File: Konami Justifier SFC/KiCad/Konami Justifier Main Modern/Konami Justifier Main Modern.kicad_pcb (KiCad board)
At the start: 4 copper layers, 25.2 x 50 mm, 20 parts, among them J1 RJ12, U1 74VHC9164FT

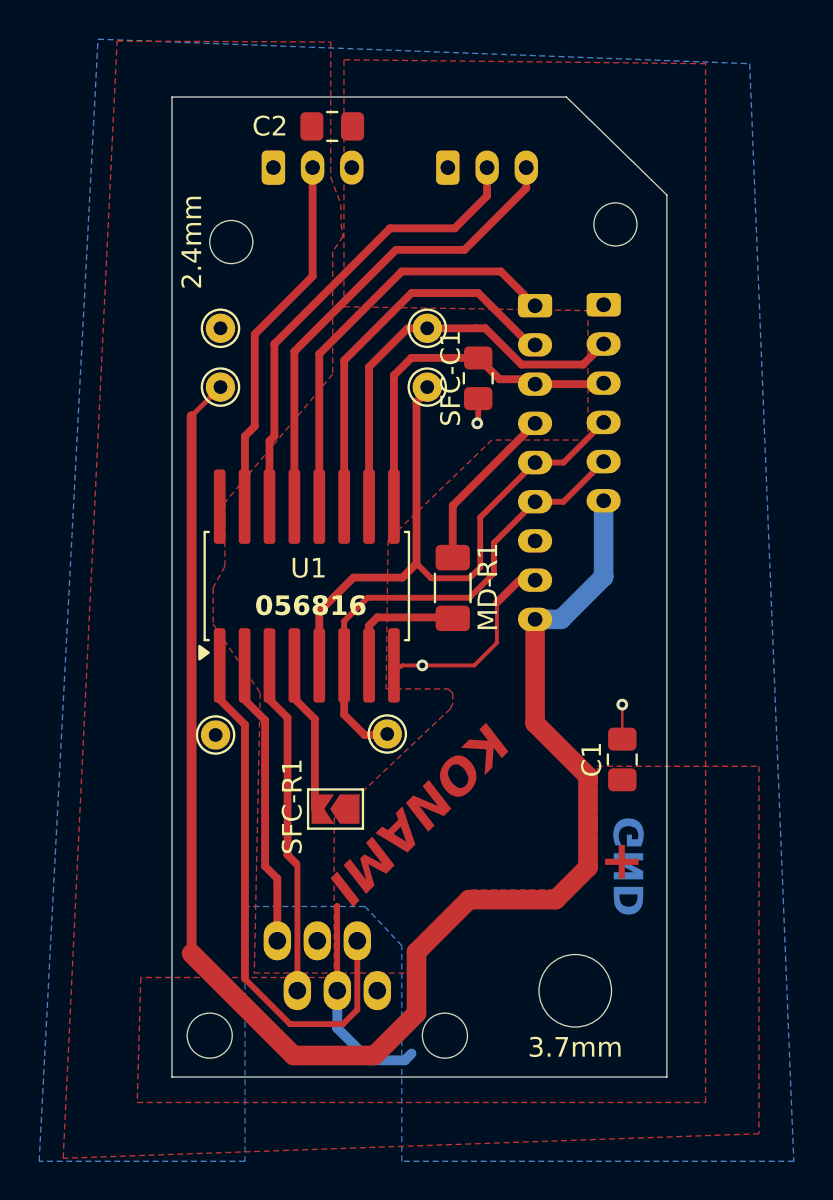
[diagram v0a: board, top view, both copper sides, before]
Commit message: Add files via upload
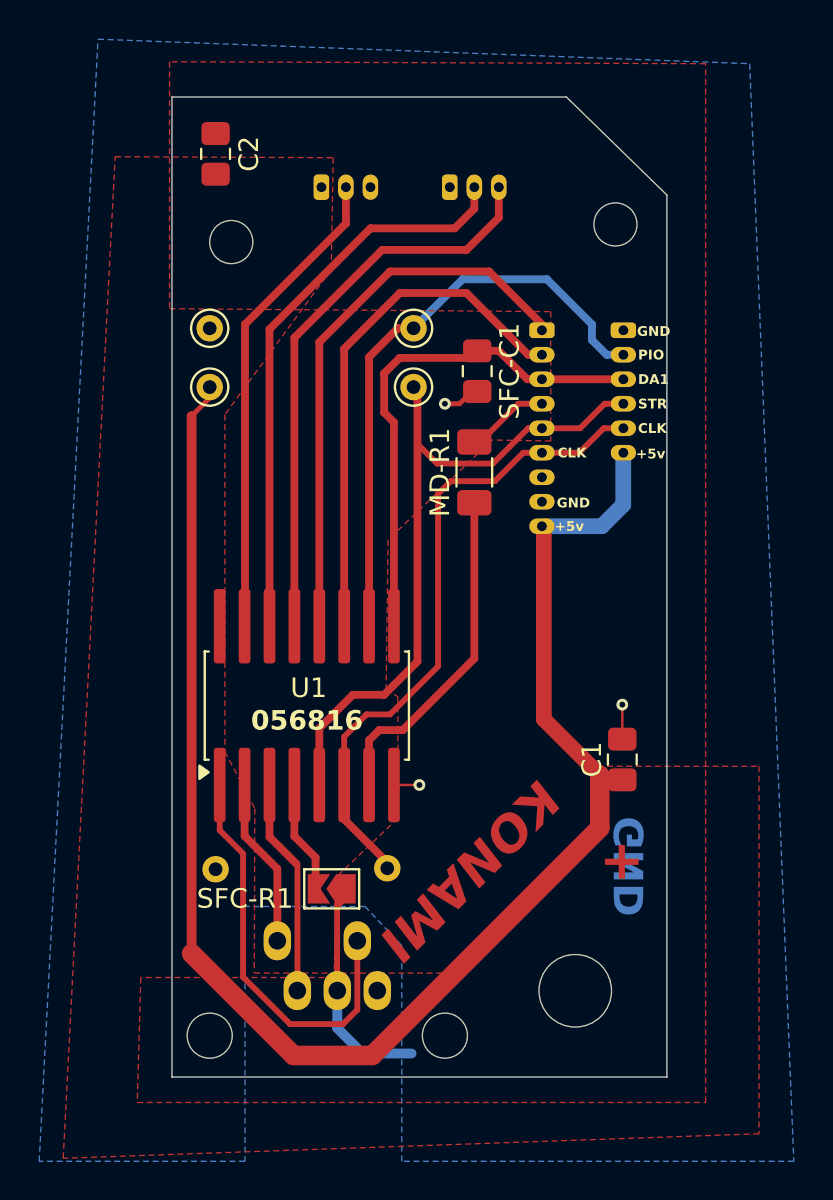
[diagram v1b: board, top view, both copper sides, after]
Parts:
- J_BTN1, J_IR1: footprint Connector_JST:JST_PH_B3B-PH-K_1x03_P2.00mm_Vertical -> Connector_Molex:Molex_PicoBlade_53048-0310_1x03_P1.25mm_Horizontal
- MD1: footprint Connector_JST:JST_PH_B9B-PH-K_1x09_P2.00mm_Vertical -> Connector_Molex:Molex_PicoBlade_53047-0910_1x09_P1.25mm_Vertical
- SFC-TP5, SFC-TP6: moved to B.Cu
- SFC1: footprint Connector_JST:JST_PH_B6B-PH-K_1x06_P2.00mm_Vertical -> Connector_Molex:Molex_PicoBlade_53047-0610_1x06_P1.25mm_Vertical
- moved SFC-TP5 6.85 mm to (142.0, 116.1), turned to 180 degrees
- moved SFC-TP6 6.85 mm to (150.8, 116.0), turned to 180 degrees
- moved C2 6.11 mm to (142.0, 79.6), turned to 90 degrees
- moved U1 6.10 mm to (146.7, 107.8)
- moved MD-R1 6.00 mm to (155.2, 95.8)
- moved SFC-R1 4.07 mm to (147.9, 117.1)
- moved J_IR1 2.65 mm to (147.4, 81.3)
- moved SFC1 1.64 mm to (162.8, 88.6)
- moved MD1 1.30 mm to (158.7, 88.6)
- moved J_BTN1 1.00 mm to (153.9, 81.3)
- moved SFC-TP1 0.70 mm to (152.1, 88.5)
- moved SFC-TP2 0.70 mm to (152.1, 91.5)
- moved SFC-TP3 0.55 mm to (141.7, 88.5)
- moved SFC-TP4 0.55 mm to (141.7, 91.5)
- moved SFC-C1 0.37 mm to (155.3, 90.7)
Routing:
- net Net-(U1-Q/D3): track 5.57 -> 16.2 mm
- net Net-(SFC1-Pin_2): track 21.9 -> 31.6 mm
- net Net-(MD1-Pin_6): track 24.9 -> 33.6 mm
- net Net-(MD1-Pin_3): track 19.5 -> 27.6 mm
- net Net-(MD1-Pin_1): track 22.1 -> 29.6 mm
- net Net-(MD1-Pin_2): track 21.5 -> 27.7 mm
- net Net-(U1-~{CLR_LOAD}): track 15.7 -> 9.55 mm
- net Net-(U1-SI): track 18.1 -> 12.0 mm
- net Net-(U1-P/S_CONT): track 27.7 -> 21.6 mm
- net Net-(J_IR1-Pin_2): track 19.5 -> 25.3 mm
- net GND: track 24.1 -> 18.3 mm
- net Net-(J_BTN1-Pin_2): track 24.6 -> 30.0 mm
- net Net-(J_BTN1-Pin_3): track 25.1 -> 30.1 mm
- net Net-(MD1-Pin_4): track 8.60 -> 4.56 mm
- net Net-(MD1-Pin_5): track 31.9 -> 35.7 mm
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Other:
- board text added: "+5v"
- board text added: "CLK"
- board text added: "DA1"
- board text added: "PIO"
- board text added: "STR"
